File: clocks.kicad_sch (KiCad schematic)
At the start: 1 part, among them U10 Si5351C-B-GM

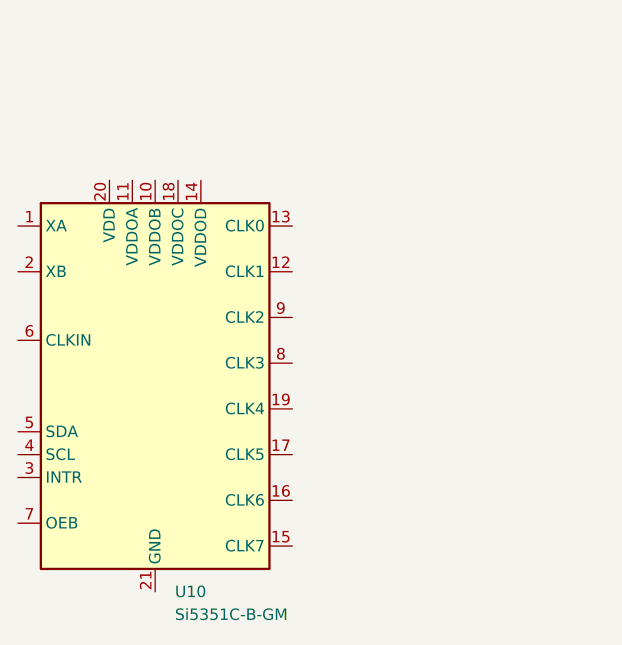
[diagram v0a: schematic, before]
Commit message: Minor updates
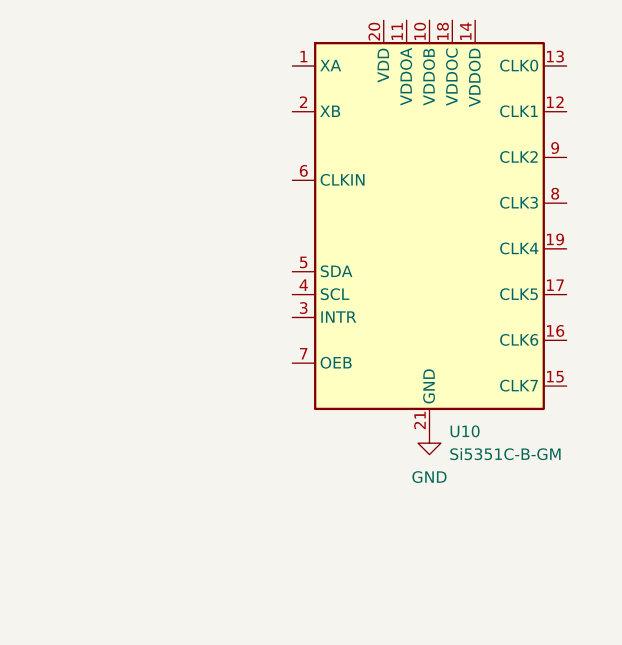
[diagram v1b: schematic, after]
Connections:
- net GND: now reaches U10.21 (GND)
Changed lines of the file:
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@@
 	(paper "A4")
 	(symbol
-		(lib_id "Oscillator:Si5351C-B-GM")
-		(at 85.09 87.63 0)
+		(lib_id "power:GND")
+		(at 115.57 92.71 0)
 		(unit 1)
 		(exclude_from_sim no)
@@
 		(on_board yes)
 		(dnp no)
+		(fields_autoplaced yes)
+		(property "Reference" "#PWR058"
+			(at 115.57 99.06 0)
+			(effects
+				(font
+					(size 1.27 1.27)
+				)
+				(hide yes)
+			)
+		)
+		(property "Value" "GND"
+			(at 115.57 97.79 0)
+			(effects
+				(font
+					(size 1.27 1.27)
+				)
+			)
+		)
+		(property "Footprint" ""
+			(at 115.57 92.71 0)
+			(effects
+				(font
+					(size 1.27 1.27)
+				)
+				(hide yes)
+			)
+		)
+		(property "Datasheet" ""
+			(at 115.57 92.71 0)
+			(effects
+				(font
+					(size 1.27 1.27)
+				)
+				(hide yes)
+			)
+		)
+		(property "Description" "Power symbol creates a global label with name \"GND\" , ground"
+			(at 115.57 92.71 0)
+			(effects
+				(font
+					(size 1.27 1.27)
+				)
+				(hide yes)
+			)
+		)
+		(pin "1"
+		)
+		(instances
+			(project ""
+				(path "/b16dfd04-6bfc-4d2d-ba2c-9a843d57dfb1/bef03a1a-2df5-41e5-bcca-109c5f92fdce"
+					(reference "#PWR058")
+					(unit 1)
+				)
+			)
+		)
+	)
+	(symbol
+		(lib_id "Oscillator:Si5351C-B-GM")
+		(at 115.57 69.85 0)
+		(unit 1)
+		(exclude_from_sim no)
+		(in_bom yes)
+		(on_board yes)
+		(dnp no)
+		(fields_autoplaced yes)
 		(property "Reference" "U10"
-			(at 87.2841 110.49 0)
+			(at 117.7641 92.71 0)
 			(effects
 				(font
@@
 		)
 		(property "Value" "Si5351C-B-GM"
-			(at 87.2841 113.03 0)
+			(at 117.7641 95.25 0)
 			(effects
 				(font
@@
 		)
 		(property "Footprint" "Package_DFN_QFN:QFN-20-1EP_4x4mm_P0.5mm_EP2.7x2.7mm"
-			(at 85.09 118.11 0)
+			(at 115.57 100.33 0)
 			(effects
 				(font
@@
 		)
 		(property "Datasheet" "https://www.silabs.com/documents/public/data-sheets/Si5351-B.pdf"
-			(at 85.09 87.63 0)
+			(at 115.57 69.85 0)
 			(effects
 				(font
@@
 		)
 		(property "Description" "I2C Programmable Any-Frequency CMOS Clock Generator, QFN-20"
-			(at 85.09 87.63 0)
+			(at 115.57 69.85 0)
 			(effects
 				(font
@@
 			)
 		)
-		(pin "2"
-		)
-		(pin "21"
-		)
-		(pin "8"
-		)
-		(pin "10"
-		)
-		(pin "1"
-		)
-		(pin "18"
-		)
-		(pin "19"
-		)
-		(pin "11"
-		)
-		(pin "17"
-		)
-		(pin "16"
+		(pin "20"
 		)
 		(pin "9"
@@
 		(pin "12"
 		)
+		(pin "18"
+		)
+		(pin "14"
+		)
+		(pin "16"
+		)
 		(pin "3"
+		)
+		(pin "15"
+		)
+		(pin "17"
+		)
+		(pin "4"
+		)
+		(pin "2"
+		)
+		(pin "10"
+		)
+		(pin "7"
+		)
+		(pin "19"
+		)
+		(pin "8"
+		)
+		(pin "21"
+		)
+		(pin "6"
+		)
+		(pin "1"
+		)
+		(pin "11"
+		)
+		(pin "13"
 		)
 		(pin "5"
 		)
-		(pin "4"
-		)
-		(pin "7"
-		)
-		(pin "6"
-		)
-		(pin "14"
-		)
-		(pin "15"
-		)
-		(pin "20"
-		)
-		(pin "13"
-		)
 		(instances
-			(project "albert"
+			(project ""
 				(path "/b16dfd04-6bfc-4d2d-ba2c-9a843d57dfb1/bef03a1a-2df5-41e5-bcca-109c5f92fdce"
 					(reference "U10")
